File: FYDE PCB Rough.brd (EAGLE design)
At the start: 73.9 x 65.7 mm, 4 parts, among them P1 SEN-11574, U1 MCU-MCP3008-I/P(DIP16-7.62MM), X1 RASPI_BOARD_B+_HDC

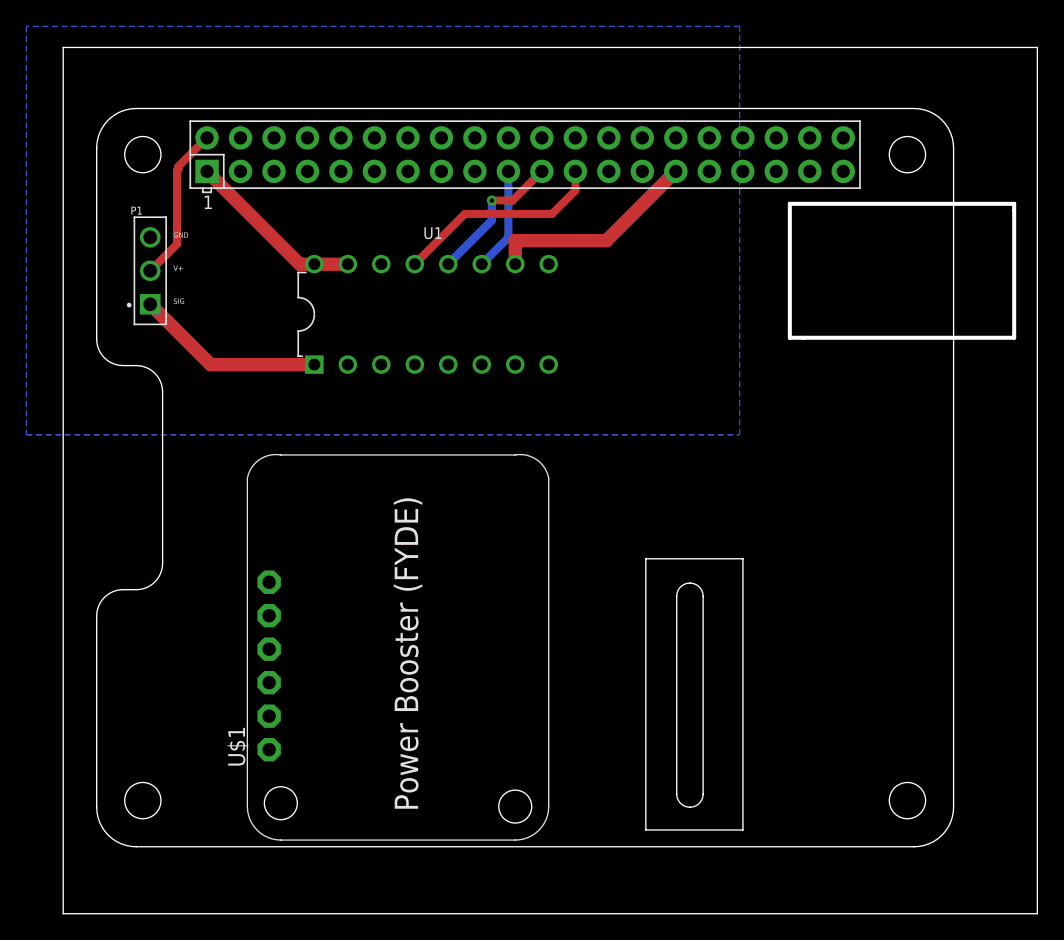
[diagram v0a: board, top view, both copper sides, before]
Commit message: Add files via upload
now with holes!
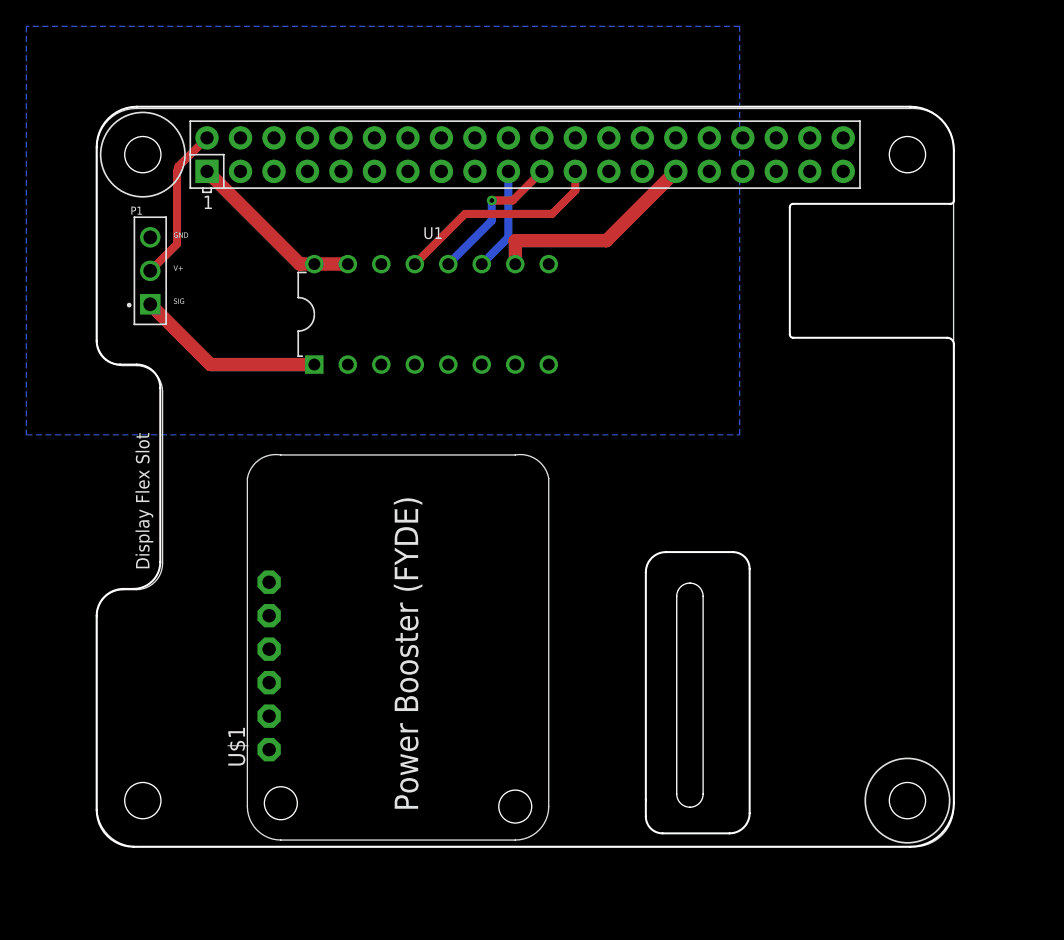
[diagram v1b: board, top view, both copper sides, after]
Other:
- board size 73.9 x 65.7 mm -> 65 x 56.1 mm
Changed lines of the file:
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@@
 <board>
 <plain>
-<wire x1="0" y1="0" x2="73.894" y2="0" width="0" layer="20"/>
-<wire x1="73.894" y1="0" x2="73.894" y2="65.71" width="0" layer="20"/>
-<wire x1="73.894" y1="65.71" x2="0" y2="65.71" width="0" layer="20"/>
-<wire x1="0" y1="65.71" x2="0" y2="0" width="0" layer="20"/>
 <dimension x1="-16.129" y1="-139.7" x2="-9.906" y2="-116.967" x3="-29.083" y3="-128.3335" textsize="1.778" layer="47" dtype="vertical" unit="inch"/>
-<polygon width="0.3048" layer="20">
-<vertex x="55.118" y="53.848"/>
-<vertex x="72.136" y="53.848"/>
-<vertex x="72.136" y="53.34"/>
-<vertex x="72.136" y="43.688"/>
-<vertex x="56.134" y="43.688"/>
-<vertex x="55.118" y="43.688"/>
-</polygon>
-<rectangle x1="44.196" y1="6.35" x2="51.562" y2="26.924" layer="20"/>
+<wire x1="2.54" y1="58.166" x2="5.588" y2="61.214" width="0.1524" layer="20" curve="-90"/>
+<wire x1="5.588" y1="61.214" x2="64.262" y2="61.214" width="0.1524" layer="20"/>
+<wire x1="64.262" y1="61.214" x2="67.564" y2="57.912" width="0.1524" layer="20" curve="-90"/>
+<wire x1="67.564" y1="57.912" x2="67.564" y2="54.102" width="0.1524" layer="20"/>
+<wire x1="67.564" y1="54.102" x2="67.31" y2="53.848" width="0.1524" layer="20" curve="-90"/>
+<wire x1="67.31" y1="53.848" x2="55.372" y2="53.848" width="0.1524" layer="20"/>
+<wire x1="55.372" y1="53.848" x2="55.118" y2="53.594" width="0.1524" layer="20" curve="90"/>
+<wire x1="55.118" y1="53.594" x2="55.118" y2="43.942" width="0.1524" layer="20"/>
+<wire x1="55.118" y1="43.942" x2="55.372" y2="43.688" width="0.1524" layer="20" curve="90"/>
+<wire x1="55.372" y1="43.688" x2="67.056" y2="43.688" width="0.1524" layer="20"/>
+<wire x1="67.056" y1="43.688" x2="67.564" y2="43.18" width="0.1524" layer="20" curve="-90"/>
+<wire x1="67.564" y1="43.18" x2="67.564" y2="8.382" width="0.1524" layer="20"/>
+<wire x1="67.564" y1="8.382" x2="64.262" y2="5.08" width="0.1524" layer="20" curve="-90"/>
+<wire x1="64.262" y1="5.08" x2="5.334" y2="5.08" width="0.1524" layer="20"/>
+<wire x1="5.334" y1="5.08" x2="2.54" y2="7.874" width="0.1524" layer="20" curve="-90"/>
+<wire x1="2.54" y1="7.874" x2="2.54" y2="22.606" width="0.1524" layer="20"/>
+<wire x1="2.54" y1="22.606" x2="4.572" y2="24.638" width="0.1524" layer="20" curve="-90"/>
+<wire x1="4.572" y1="24.638" x2="5.334" y2="24.638" width="0.1524" layer="20"/>
+<wire x1="5.334" y1="24.638" x2="7.366" y2="26.67" width="0.1524" layer="20" curve="90"/>
+<wire x1="7.366" y1="26.67" x2="7.366" y2="39.878" width="0.1524" layer="20"/>
+<wire x1="7.366" y1="39.878" x2="5.588" y2="41.656" width="0.1524" layer="20" curve="90"/>
+<wire x1="5.588" y1="41.656" x2="4.318" y2="41.656" width="0.1524" layer="20"/>
+<wire x1="4.318" y1="41.656" x2="2.54" y2="43.434" width="0.1524" layer="20" curve="-90"/>
+<wire x1="2.54" y1="43.434" x2="2.54" y2="58.166" width="0.1524" layer="20"/>
+<wire x1="44.196" y1="8.636" x2="44.196" y2="25.908" width="0.1524" layer="20"/>
+<wire x1="44.196" y1="25.908" x2="45.72" y2="27.432" width="0.1524" layer="20" curve="-90"/>
+<wire x1="45.72" y1="27.432" x2="50.8" y2="27.432" width="0.1524" layer="20"/>
+<wire x1="50.8" y1="27.432" x2="52.07" y2="26.162" width="0.1524" layer="20" curve="-90"/>
+<wire x1="52.07" y1="26.162" x2="52.07" y2="7.62" width="0.1524" layer="20"/>
+<wire x1="52.07" y1="7.62" x2="50.546" y2="6.096" width="0.1524" layer="20" curve="-90"/>
+<wire x1="50.546" y1="6.096" x2="45.466" y2="6.096" width="0.1524" layer="20"/>
+<wire x1="45.466" y1="6.096" x2="44.196" y2="7.366" width="0.1524" layer="20" curve="-90"/>
+<wire x1="44.196" y1="7.366" x2="44.196" y2="8.636" width="0.1524" layer="20"/>
 </plain>
 <attributes>
